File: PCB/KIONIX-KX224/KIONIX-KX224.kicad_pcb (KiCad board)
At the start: 2 copper layers, 11 parts, among them J1 Conn_01x01, J2 Conn_01x01, J3 Conn_01x01, J4 Conn_01x01, J5 Conn_01x01, J6 Conn_01x01

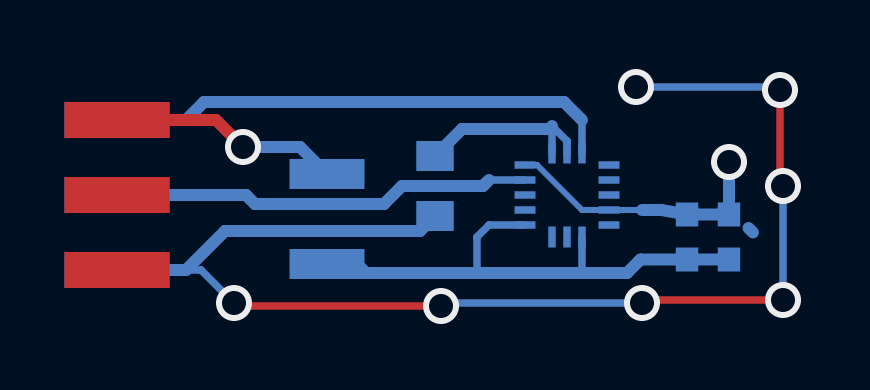
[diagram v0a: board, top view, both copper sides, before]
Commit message: PCB - Kionix v 1.5, ready to print
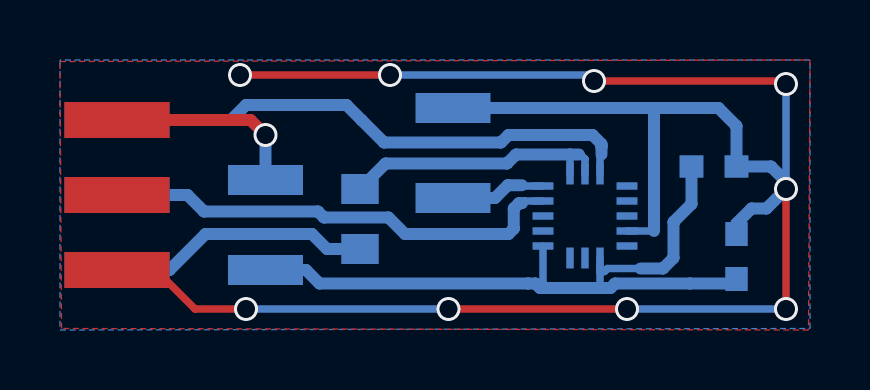
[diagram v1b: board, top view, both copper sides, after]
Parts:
- added JP3: Jumper, Capacitors_SMD:C_1210, B.Cu at (140.1, 93.1)
- moved JP1 2.73 mm to (137.0, 95.3)
- moved C1 2.40 mm to (148.8, 93.5), turned to 0 degrees
- moved JP2 2.06 mm to (133.8, 95.5)
- moved C2 1.77 mm to (149.6, 96.5)
- moved Kx1 0.92 mm to (144.5, 95.2)
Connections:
- Kx1 pad 10: (no net) -> Net-(Kx1-Pad10)
- Kx1 pad 11: (no net) -> Net-(Kx1-Pad11)
- Kx1 pad 13: (no net) -> Net-(Kx1-Pad13)
- Kx1 pad 15: (no net) -> Net-(Kx1-Pad15)
- Kx1 pad 16: (no net) -> Net-(Kx1-Pad16)
- Kx1 pad 2: (no net) -> Net-(Kx1-Pad2)
- Kx1 pad 3: (no net) -> Net-(Kx1-Pad3)
- Kx1 pad 5: GNDREF -> Net-(JP3-Pad2)
- Kx1 pad 9: (no net) -> Net-(Kx1-Pad9)
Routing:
- net GNDREF: track 9.28 -> 69.3 mm, vias 1 -> 9
- net Net-(J6-Pad1): track 46.1 -> 8.80 mm, vias 7 -> 0
- net /VDD: track 18.6 -> 25.1 mm
- net Net-(JP3-Pad2): track 0.00 -> 3.19 mm
- net /Miso/Mosi: track 6.38 -> 9.19 mm
- net /SCLK: track 14.1 -> 16.2 mm
- net Net-(J1-Pad1): track 7.75 -> 9.46 mm
- net /CS/SCL: track 18.6 -> 19.6 mm
- added copper zone on B.Cu, net GNDREF
- added copper zone on F.Cu, net GNDREF
